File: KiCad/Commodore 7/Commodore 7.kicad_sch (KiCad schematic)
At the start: 18 parts, among them J2 Conn_02x20_Odd_Even_MountingP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, U1 IIM-42652 Main Accelerometer, U2 Barometer, U3 IIM-42652 - Main Acceleromete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, U4 BMI270 - Secondary Accelerome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, U5 MMC5983MA, U6 TMP1075D, U7 TCA9543APWR

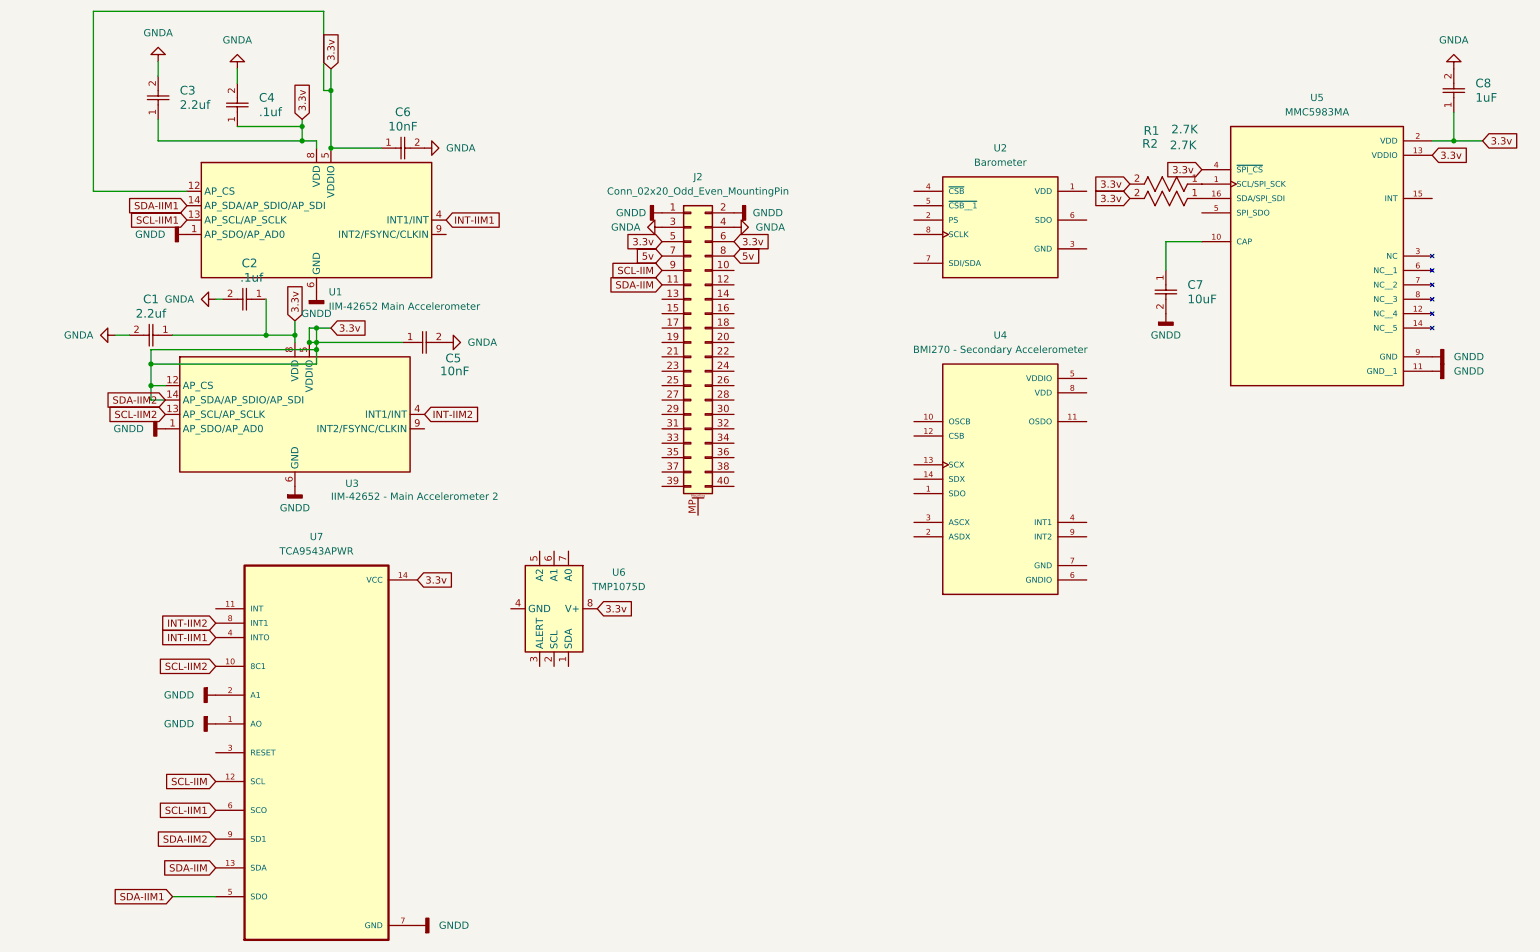
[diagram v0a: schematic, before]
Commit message: connecting 6 or 7 wires ha ha ha ha ha ha ha
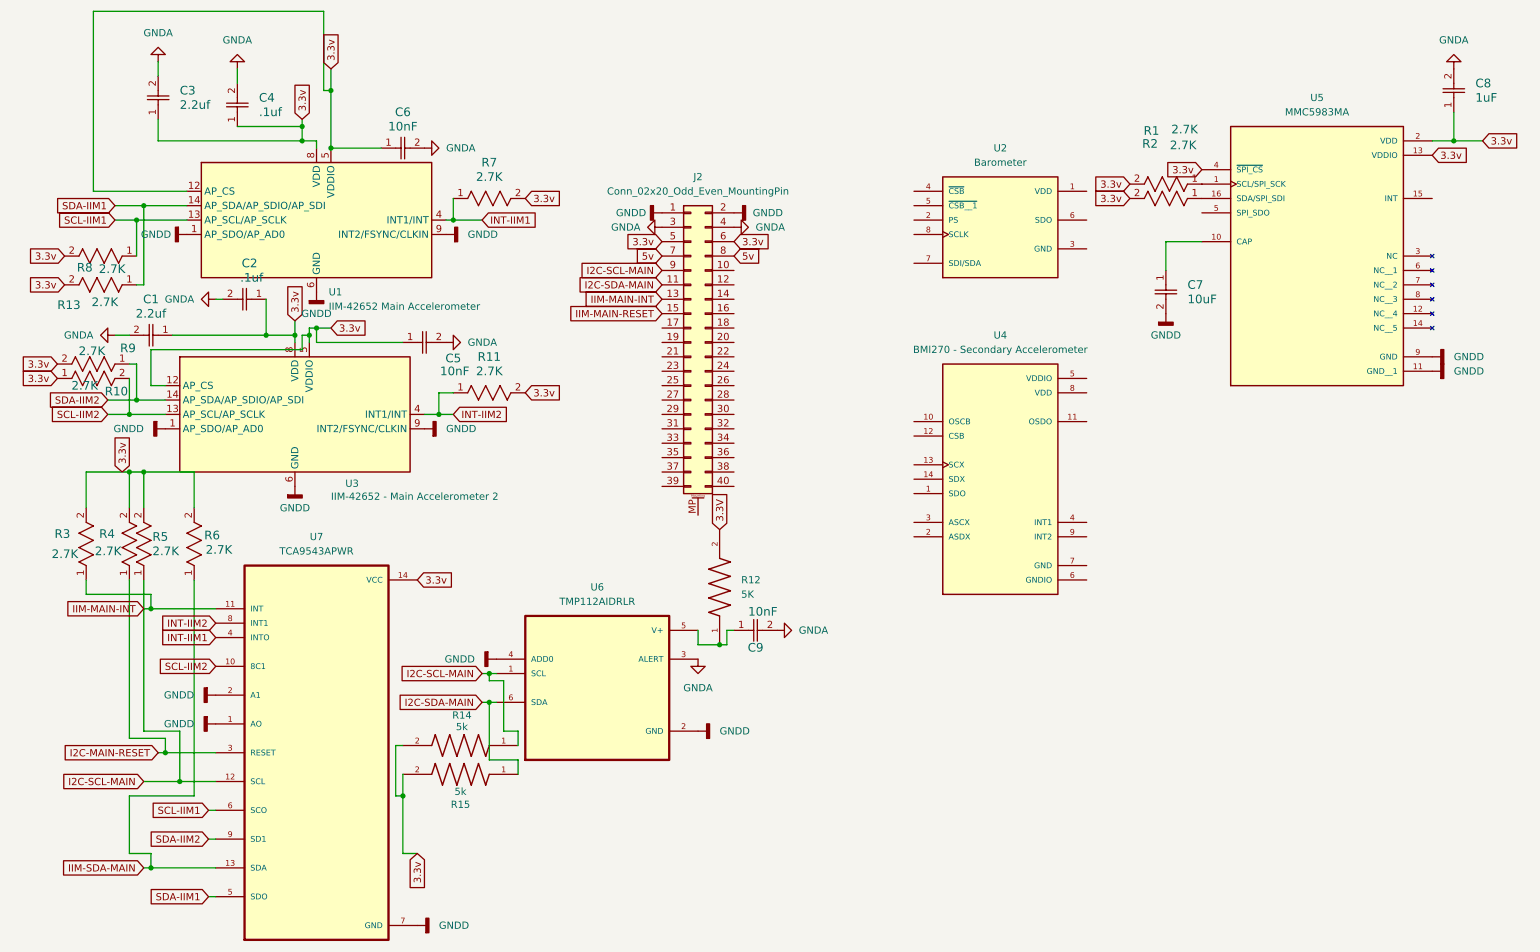
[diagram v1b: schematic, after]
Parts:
- removed U6: TMP1075D, Package_SO:SO-8_3.9x4.9mm_P1.27mm, symbol Sensor_Temperature:TMP1075D
- added C9: 10nF, C0603C103K4RECTU:CAPC17595_87N_KEM, symbol 2025-10-06_19-30-10:C0603C103K4RECTU
- added R10, R11, R13, R3, R4, R5, R6, R7, R8, R9: 2.7K, CRG0805F2K7:RES0805_CRG_TYCO_TYC, symbol 2025-10-06_20-52-39:CRG0805F2K7
- added R12: 5K, CRCW08055K00FKTA:RESC2012X50N, symbol CRCW08055K00FKTA:CRCW08055K00FKTA
- added R14, R15: 5k, CRCW08055K00FKTA:RESC2012X50N, symbol CRCW08055K00FKTA:CRCW08055K00FKTA
- added U6: TMP112AIDRLR, TMP112AIDRLR:SOT50P160X60-6N, symbol TMP112AIDRLR:TMP112AIDRLR
- C8: footprint YAG_CC0603_YAG -> CC0603KRX7R7BB105:YAG_CC0603_YAG
- R1, R2: footprint RES0805_CRG_TYCO_TYC -> CRG0805F2K7:RES0805_CRG_TYCO_TYC
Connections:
- net SCL-IIM is gone; now on net I2C-SCL-MAIN: J2.9 (Pin_9), U7.12 (SCL)
- net 3.3v: now also R10.1, R11.2, R13.2, R14.2, R15.2, R3.2, R4.2, R5.2, R6.2, R7.2, R8.2, R9.2; no longer U3.14 (AP_SDA/AP_SDIO/AP_SDI), U7.9 (SD1)
- net GNDA: now also C9.2, U6.3 (ALERT)
- net GNDD: now also U1.9 (INT2/FSYNC/CLKIN), U3.9 (INT2/FSYNC/CLKIN), U6.2 (GND), U6.4 (ADD0)
- net INT-IIM1: now also R7.1
- net INT-IIM2: now also R11.1
- net SCL-IIM1: now also R8.1
- net SCL-IIM2: now also R10.2
- net SDA-IIM1: now also R13.1
- net I2C-SCL-MAIN: now reaches J2.13 (Pin_13)
- net I2C-SCL-MAIN: now also U7.11 (INT), R14.1, R3.1, R5.1, U6.1 (SCL)
- net IIM-MAIN-RESET: now reaches J2.15 (Pin_15)
- net I2C-MAIN-RESET: now reaches U7.3 (RESET)
- net I2C-MAIN-RESET: now also R4.1
- net SDA-IIM renamed I2C-SDA-MAIN
- net I2C-SDA-MAIN: now also R15.1, U6.6 (SDA); no longer U7.13 (SDA)
- new net: C9.1, R12.1, U6.5 (V+)
- new net 3.3V: R12.2
- new net IIM-SDA-MAIN: R6.1, U7.13 (SDA)
- new net SDA-IIM2: R9.1, U3.14 (AP_SDA/AP_SDIO/AP_SDI), U7.9 (SD1)
